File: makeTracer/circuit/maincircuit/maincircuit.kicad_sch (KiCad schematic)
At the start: 17 parts, among them IC1 PIC16F1778-I/SP, J1 PICKit3, J2 Sensor, J3 I^{2}C, J4 LED, J7 Bus_PCI_Express_x1_Debug, SW1 SW_DPDT_x2, SW2 Reset, SW3 Red, SW4 Green

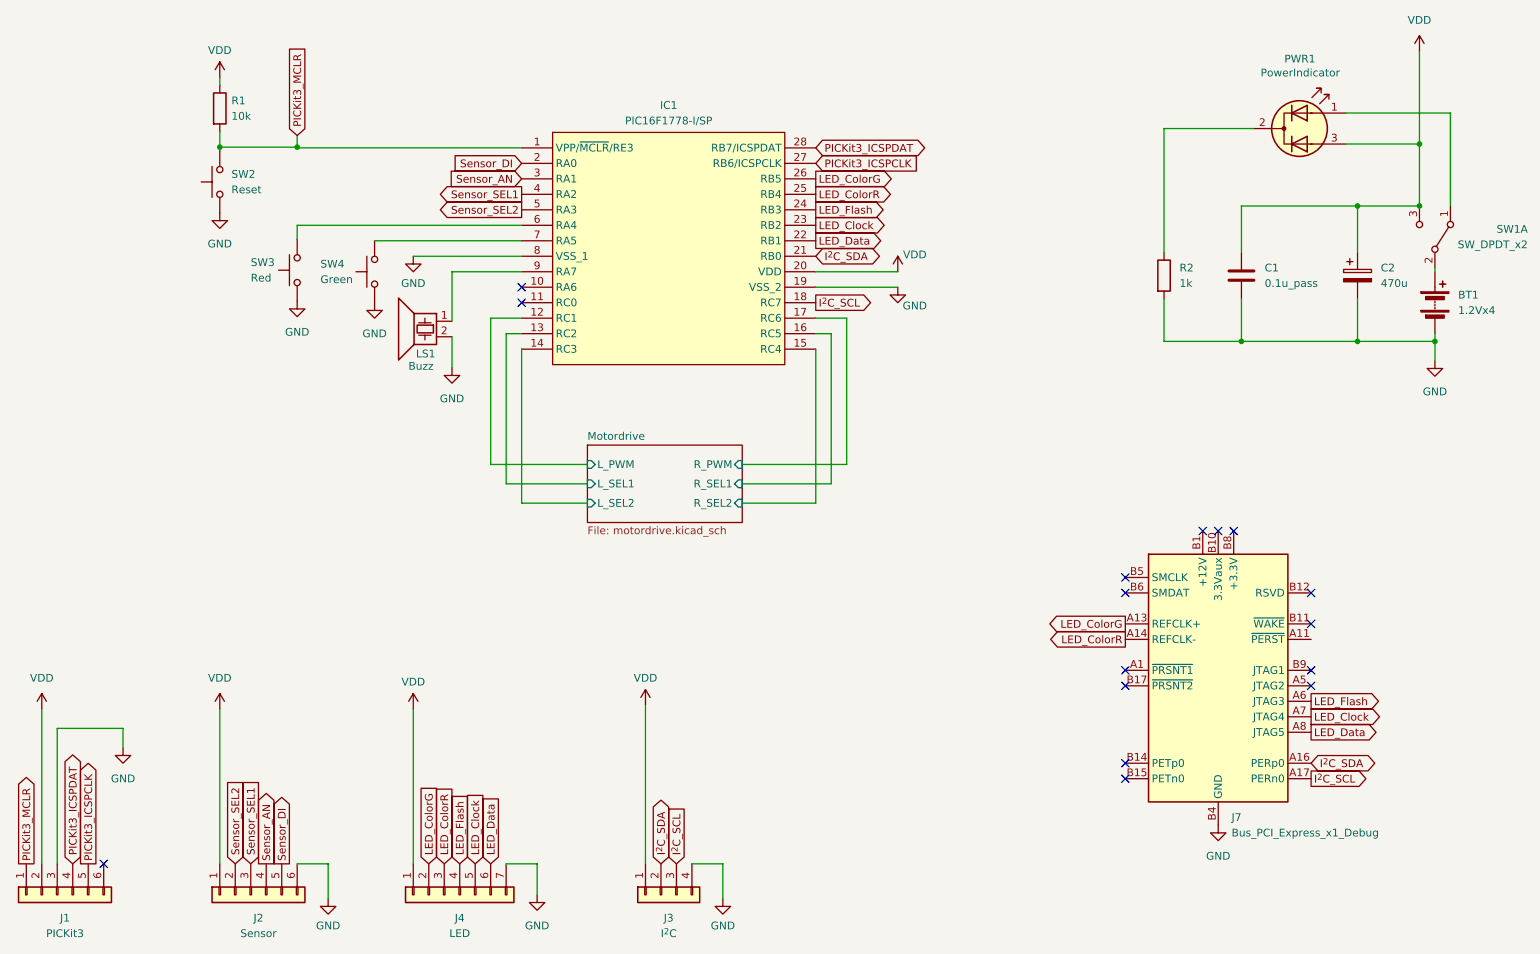
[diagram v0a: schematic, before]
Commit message: complete: circuit
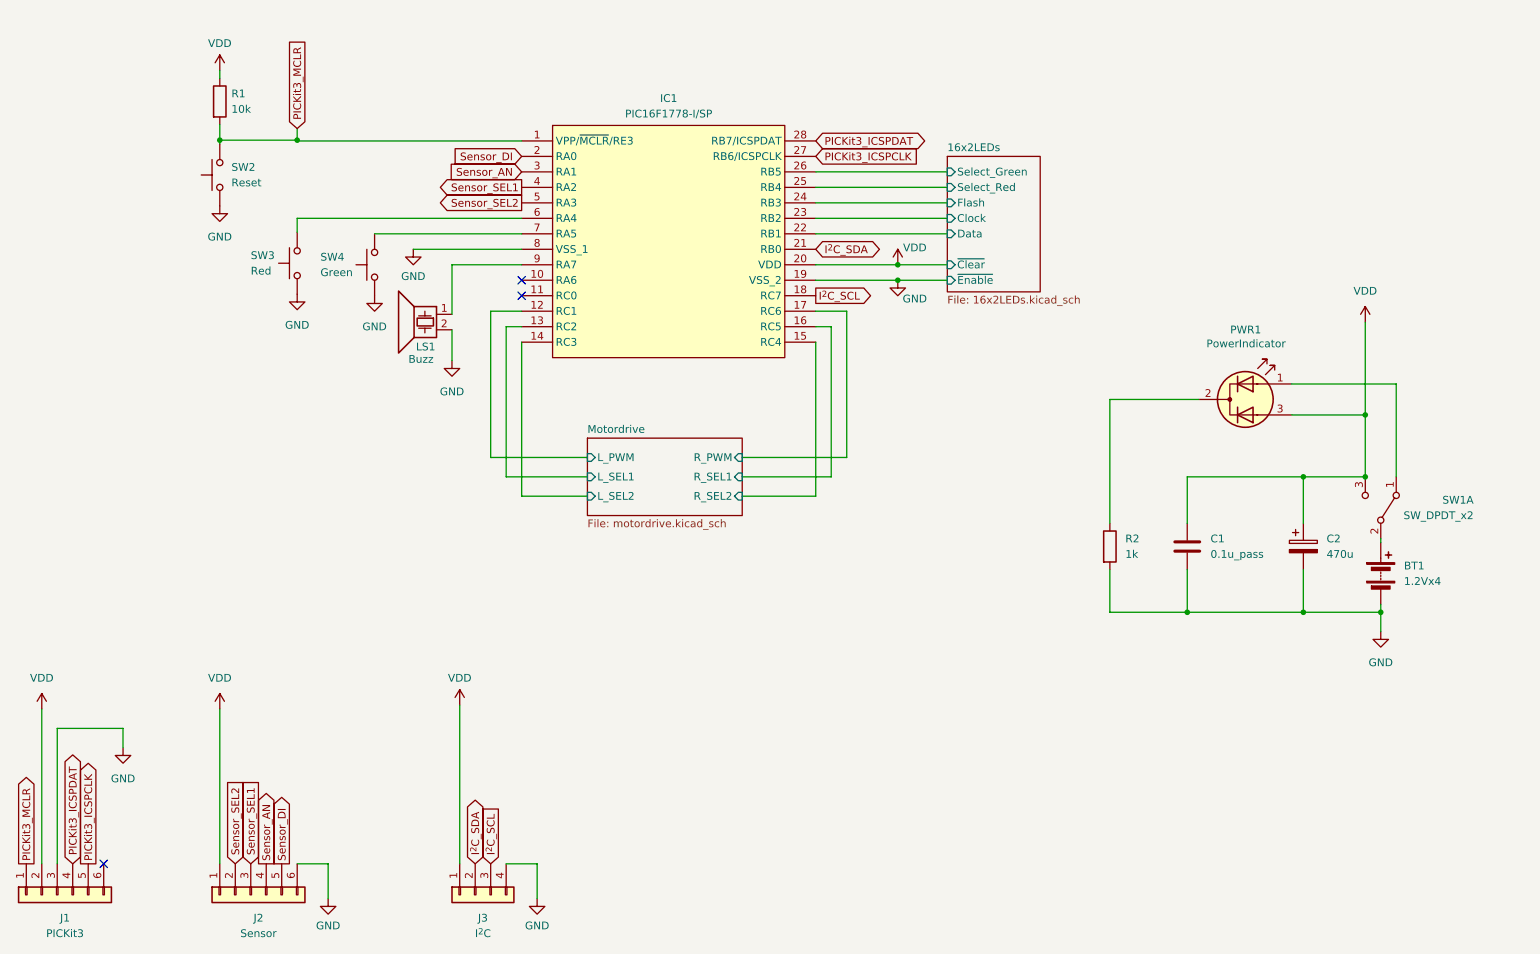
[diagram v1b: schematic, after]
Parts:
- removed J4: LED, Connector_PinHeader_2.54mm:PinHeader_1x07_P2.54mm_Horizontal, symbol Connector_Generic:Conn_01x07
- removed J7: Bus_PCI_Express_x1_Debug, Connector_PCBEdge:BUS_PCIexpress_x1, symbol Connector:Bus_PCI_Express_x1
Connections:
- net LED_Clock renamed 16x2LEDs/Clock
- net LED_ColorG renamed 16x2LEDs/Select_Green
- net LED_ColorR renamed 16x2LEDs/Select_Red
- net LED_Data renamed 16x2LEDs/Data
- net LED_Flash renamed 16x2LEDs/Flash
- no-connect marks 16 -> 3
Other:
- added sheet 16x2LEDs (16x2LEDs.kicad_sch)
- moved on the sheet: BT1, C1, C2, IC1, J3, LS1, PWR1, R1, R2, SW1A, SW2, SW3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
